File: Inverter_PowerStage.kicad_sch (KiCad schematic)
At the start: 5 parts, among them IC4 ISO7760FQDWQ1, J2 Conn_01x02_Pin, U10 IGCM15F60GA

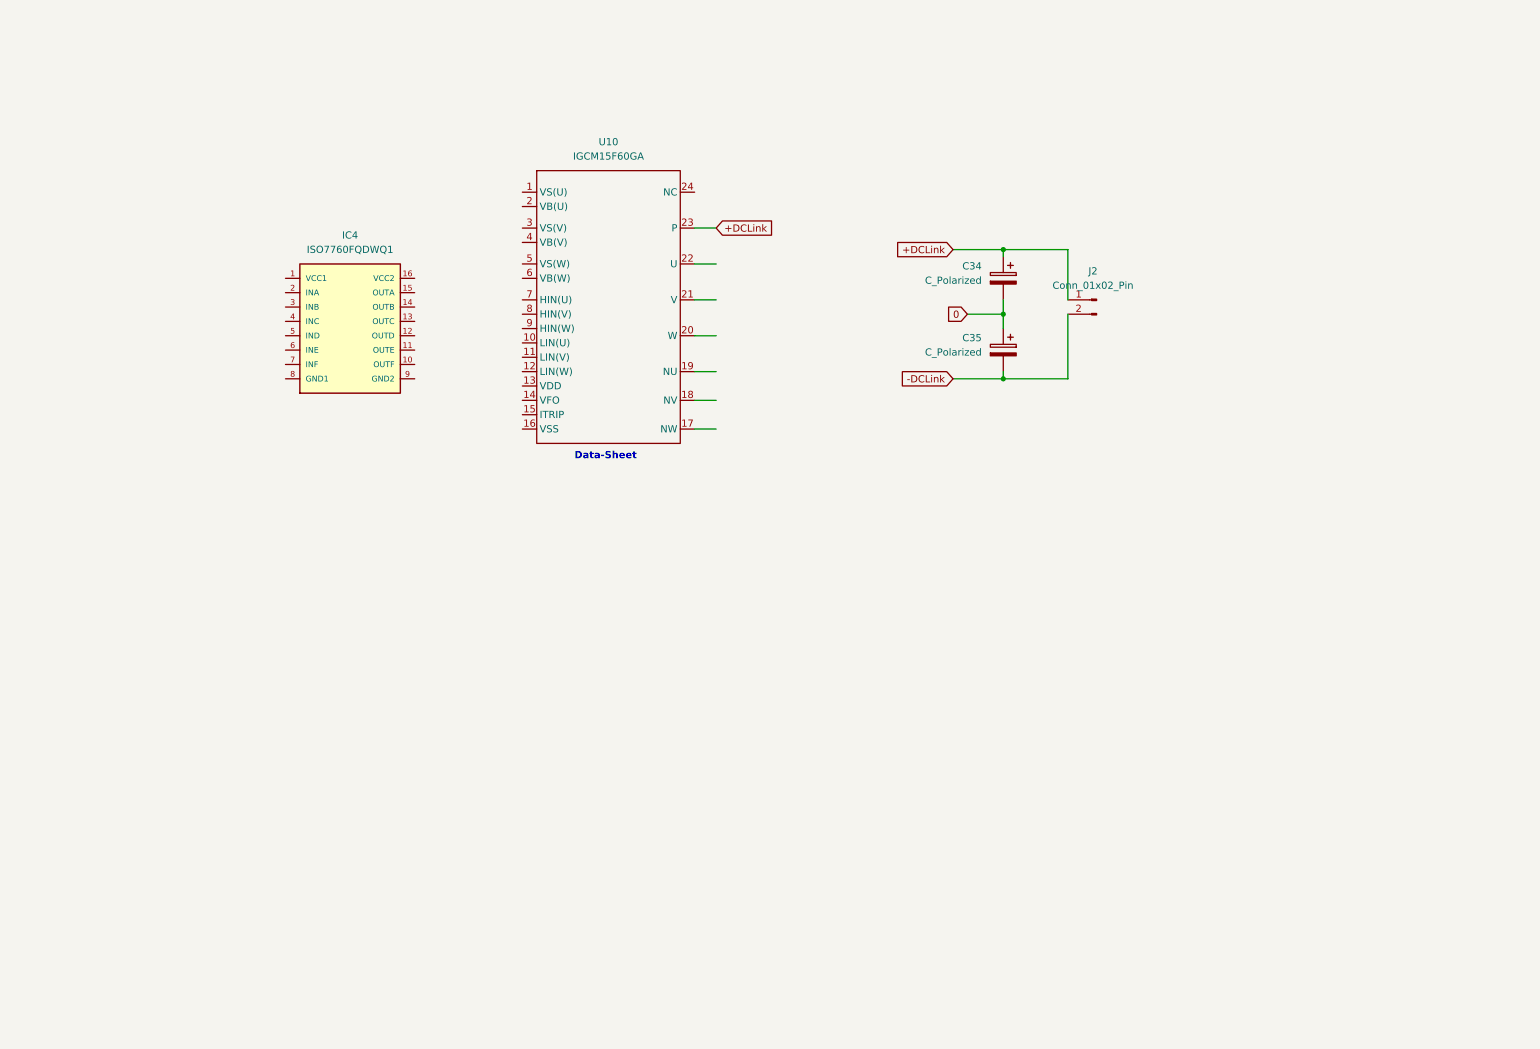
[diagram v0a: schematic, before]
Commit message: #
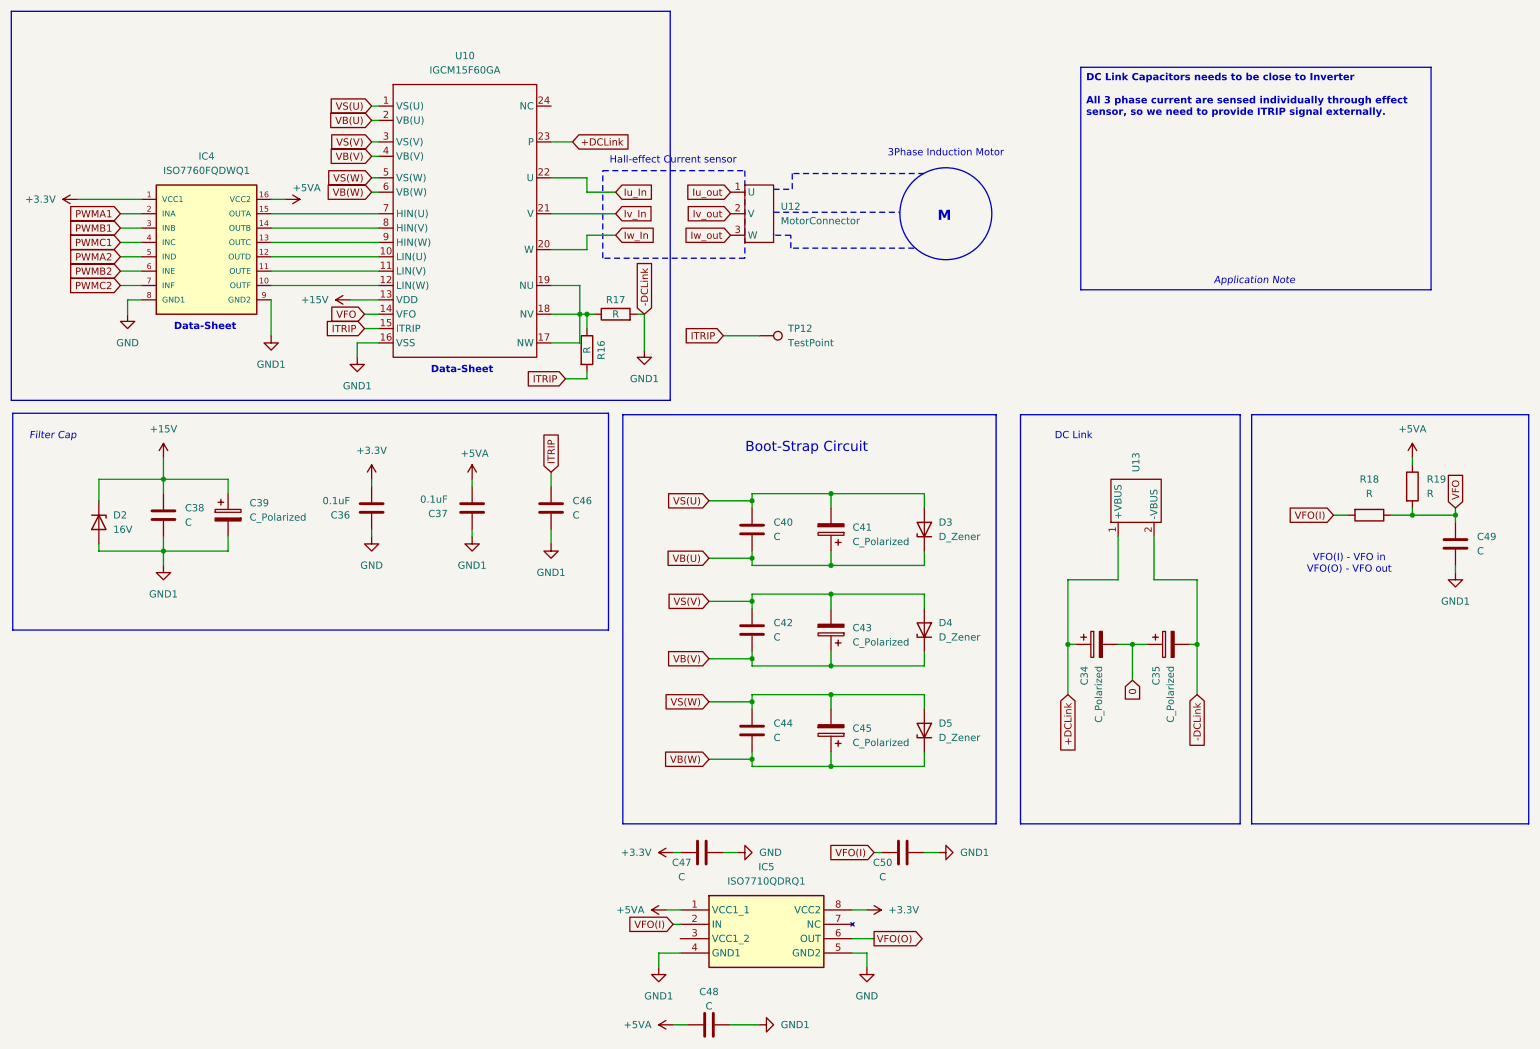
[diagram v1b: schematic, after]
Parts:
- removed J2: Conn_01x02_Pin, symbol Connector:Conn_01x02_Pin
- added C36, C37: 0.1uF, symbol Device:C
- added C38, C40, C42, C44, C46, C47, C48, C49, C50: C, symbol Device:C
- added C39, C41, C43, C45: C_Polarized, symbol Device:C_Polarized
- added D2: 16V, symbol Device:D_Zener
- added D3, D4, D5: D_Zener, symbol Device:D_Zener
- added IC5: ISO7710QDRQ1, SOIC127P600X175-8N, symbol ISO7710QDRQ1:ISO7710QDRQ1
- added R16, R17, R18, R19: R, symbol Device:R
- added TP12: TestPoint, symbol Connector:TestPoint
- added U12: MotorConnector, symbol EVInverter:MotorConnector
- added U13: (no value), symbol EVInverter:DCBus
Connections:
- net -DCLink is gone; now on net GND1: C35.2
- net +DCLink: now also U13.1 (+VBUS)
- net +3.3V: now reaches IC4.1 (VCC1)
- net +3.3V: now also C36.2, C47.1, IC5.8 (VCC2)
- net at IC4.10 (OUTF): now also U10.12 (LIN(W))
- net at IC4.11 (OUTE): now also U10.11 (LIN(V))
- net at IC4.12 (OUTD): now also U10.10 (LIN(U))
- net at IC4.13 (OUTC): now also U10.9 (HIN(W))
- net at IC4.14 (OUTB): now also U10.8 (HIN(V))
- net at IC4.15 (OUTA): now also U10.7 (HIN(U))
- net +5VA: now reaches IC4.16 (VCC2)
- net +5VA: now also C37.2, C48.1, IC5.1 (VCC1_1), R19.1
- net PWMA1: now reaches IC4.2 (INA)
- net PWMB1: now reaches IC4.3 (INB)
- net PWMC1: now reaches IC4.4 (INC)
- net PWMA2: now reaches IC4.5 (IND)
- net PWMB2: now reaches IC4.6 (INE)
- net PWMC2: now reaches IC4.7 (INF)
- net GND: now reaches IC4.8 (GND1)
- net GND: now also C36.1, C47.2, IC5.5 (GND2)
- net GND1: now reaches IC4.9 (GND2)
- net GND1: now also U10.16 (VSS), C37.1, C38.2, C39.2, C46.2, C48.2, C49.2, C50.2, D2.2 (A), IC5.4 (GND1), R17.2, U13.2 (-VBUS)
- net VS(U): now reaches U10.1 (VS(U))
- net VS(U): now also C40.1, C41.2, D3.2 (A)
- net +15V: now reaches U10.13 (VDD)
- net +15V: now also C38.1, C39.1, D2.1 (K)
- net VFO: now reaches U10.14 (VFO)
- net VFO: now also C49.1, R18.1, R19.2
- net ITRIP: now reaches U10.15 (ITRIP)
- net ITRIP: now also C46.1, R16.2, TP12.1
- net at U10.17 (NW): now also U10.18 (NV), U10.19 (NU), R16.1, R17.1
- net VB(U): now reaches U10.2 (VB(U))
- net VB(U): now also C40.2, C41.1, D3.1 (K)
- net Iw_In: now reaches U10.20 (W)
- net Iv_In: now reaches U10.21 (V)
- net Iu_In: now reaches U10.22 (U)
- net VS(V): now reaches U10.3 (VS(V))
- net VS(V): now also C42.1, C43.2, D4.2 (A)
- net VB(V): now reaches U10.4 (VB(V))
- net VB(V): now also C42.2, C43.1, D4.1 (K)
- net VS(W): now reaches U10.5 (VS(W))
- net VS(W): now also C44.1, C45.2, D5.2 (A)
- net VB(W): now reaches U10.6 (VB(W))
- net VB(W): now also C44.2, C45.1, D5.1 (K)
- new net Iu_out: U12.1 (U)
- new net Iv_out: U12.2 (V)
- new net Iw_out: U12.3 (W)
- new net VFO(I): C50.1, IC5.2 (IN), R18.2
- new net VFO(O): IC5.6 (OUT)
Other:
- note added: "3Phase Induction Motor"
- note added: "Application Note"
- note added: "Boot-Strap Circuit"
- note added: "DC Link"
- note added: "Filter Cap"
- note added: "Hall-effect Current sensor"
- note added: "M"
- note added: "VFO(I) - VFO in VFO(O) - VFO out"
- moved on the sheet: C34, C35, IC4, U10
